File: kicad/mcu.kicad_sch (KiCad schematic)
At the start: 36 parts, among them J8 USB_C_Receptacle_USB2.0_14P, J9 Conn_01x03, SW1 SW_Push, SW2 SW_Push, U12 ESP32-S3-WROOM-1-N8R2

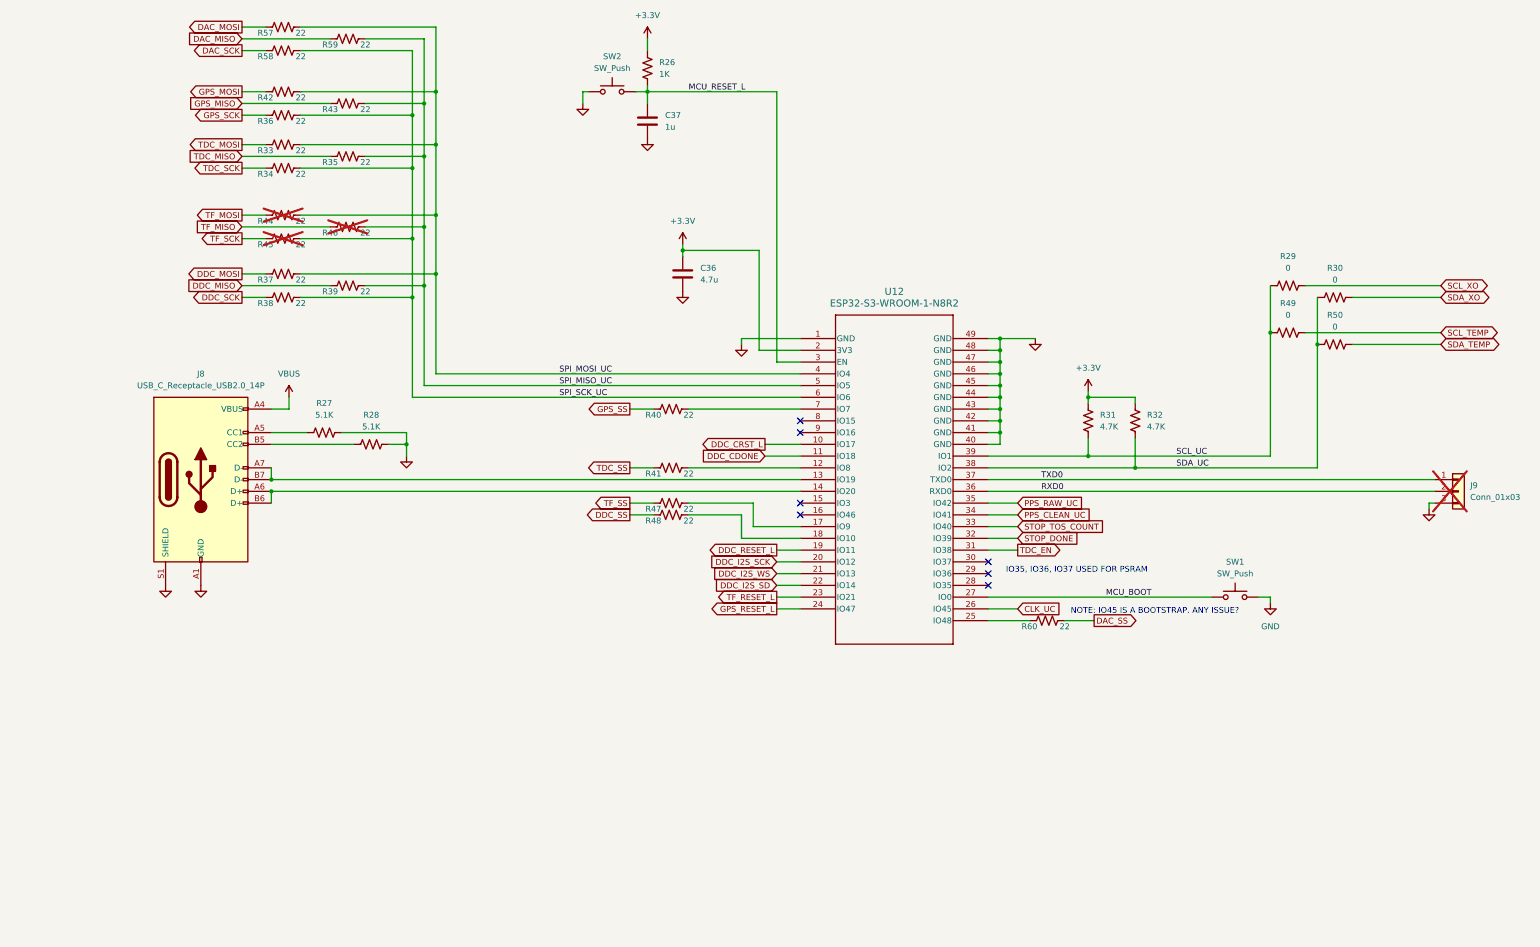
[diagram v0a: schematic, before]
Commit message: add lte radio and various fixes
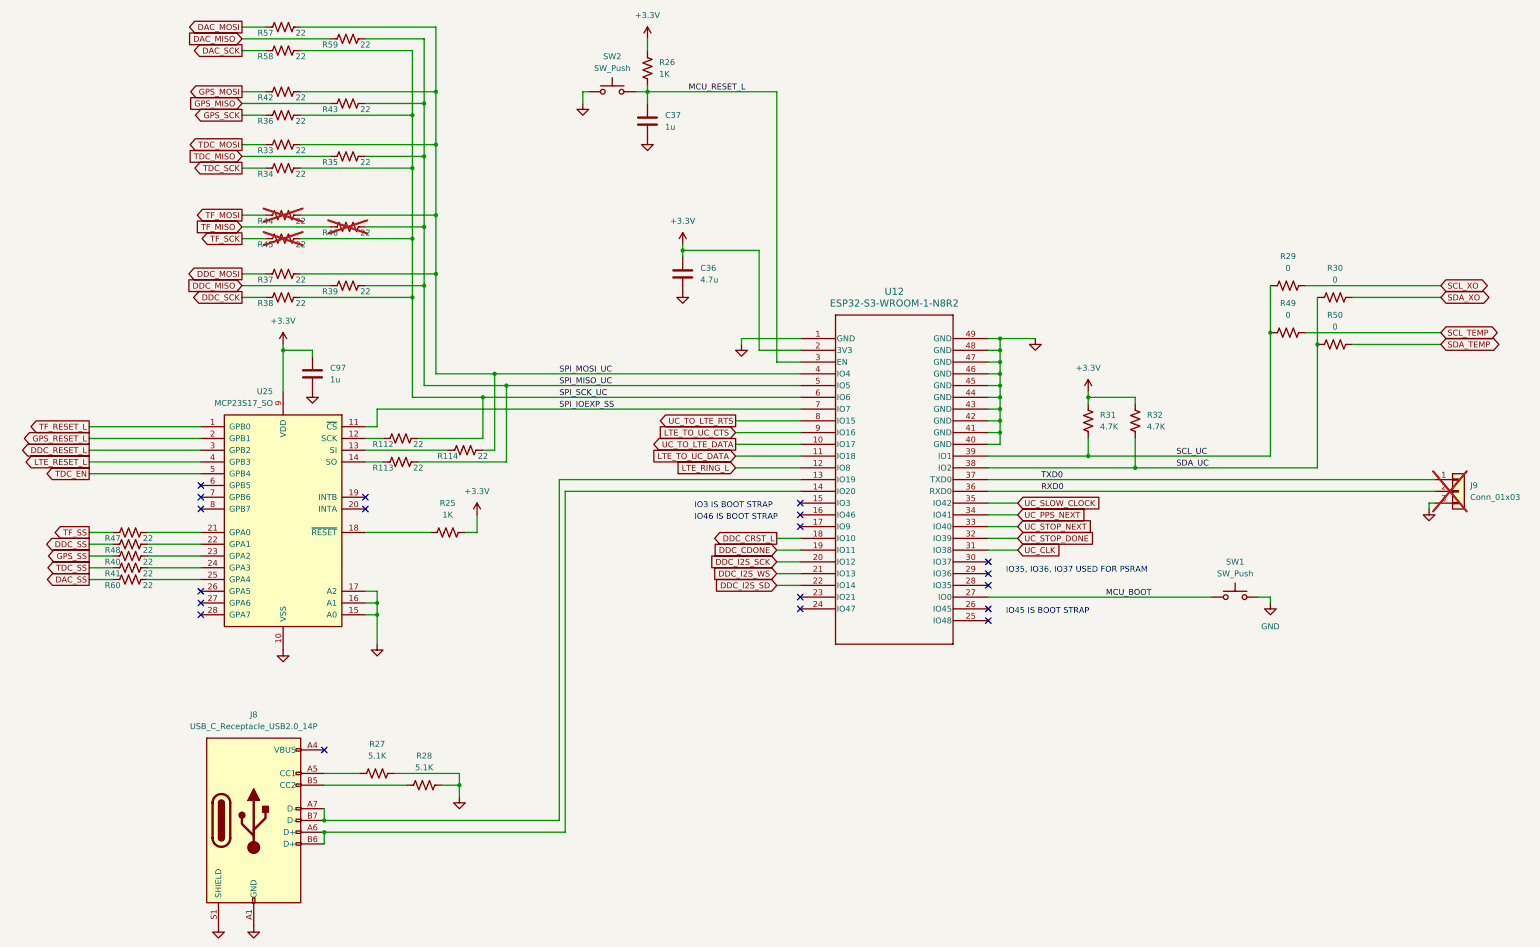
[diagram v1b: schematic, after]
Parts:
- added C97: 1u, symbol Device:C
- added R112, R113, R114: 22, symbol Device:R_US
- added R25: 1K, symbol Device:R_US
- added U25: MCP23S17_SO, Package_SO:SOIC-28W_7.5x17.9mm_P1.27mm, symbol Interface_Expansion:MCP23S17_SO
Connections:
- net +3.3V: now also C97.1, R25.2, U25.9 (VDD)
- net DDC_CDONE: now also U12.19 (IO11); no longer U12.11 (IO18)
- net DDC_CRST_L: now also U12.18 (IO10); no longer U12.10 (IO17)
- net DDC_RESET_L: now also U25.3 (GPB2); no longer U12.19 (IO11)
- net GND: now also C97.2, U25.10 (VSS), U25.15 (A0), U25.16 (A1), U25.17 (A2)
- net GPS_RESET_L: now also U25.2 (GPB1); no longer U12.24 (IO47)
- net SPI_MISO_UC: now also R113.2
- net SPI_MOSI_UC: now also R114.2
- net SPI_SCK_UC: now also R112.2
- net TDC_EN: now also U25.5 (GPB4); no longer U12.31 (IO38)
- net TF_RESET_L: now also U25.1 (GPB0); no longer U12.23 (IO21)
- net at R48.2: now also U25.22 (GPA1); no longer U12.18 (IO10)
- net at R41.2: now also U25.24 (GPA3); no longer U12.12 (IO8)
- net at U12.17 (IO9): no longer R47.2
- net at U12.25 (IO48): no longer R60.1
- net at R40.2: now also U25.23 (GPA2); no longer U12.7 (IO7)
- net UC_TO_LTE_RTS: now reaches U12.8 (IO15)
- net LTE_TO_UC_CTS: now reaches U12.9 (IO16)
- net CLK_UC: no longer names the net of U12.26 (IO45)
- net PPS_CLEAN_UC renamed UC_PPS_NEXT
- net PPS_RAW_UC renamed UC_SLOW_CLOCK
- net STOP_DONE renamed UC_STOP_DONE
- net STOP_TOS_COUNT renamed UC_STOP_NEXT
- net VBUS: no longer names the net of J8.A4 (VBUS), J8.A9 (VBUS), J8.B4 (VBUS), J8.B9 (VBUS)
- new net: R60.1, U25.25 (GPA4)
- new net: R112.1, U25.12 (SCK)
- new net: R47.2, U25.21 (GPA0)
- new net: R25.1, U25.18 (~{RESET})
- new net: R113.1, U25.14 (SO)
- new net: R114.1, U25.13 (SI)
- new net LTE_RESET_L: U25.4 (GPB3)
- new net LTE_RING_L: U12.12 (IO8)
- new net LTE_TO_UC_DATA: U12.11 (IO18)
- new net SPI_IOEXP_SS: U12.7 (IO7), U25.11 (~{CS})
- new net UC_CLK: U12.31 (IO38)
- new net UC_TO_LTE_DATA: U12.10 (IO17)
- no-connect marks 7 -> 19
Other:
- note added: "IO3 IS BOOT STRAP"
- note added: "IO45 IS BOOT STRAP"
- note added: "IO46 IS BOOT STRAP"
- note removed: "NOTE: IO45 IS A BOOTSTRAP. ANY ISSUE?"
- moved on the sheet: J8, R27, R28, R40, R41, R47, R48, R60

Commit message: assign footprints
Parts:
- C36, C37, C97: footprint (none) -> Capacitor_SMD:C_0603_1608Metric_Pad1.08x0.95mm_HandSolder
- J8: footprint (none) -> Connector_USB:USB_C_Receptacle_Molex_105450-0101
- J9: footprint (none) -> Connector_PinHeader_2.54mm:PinHeader_1x03_P2.54mm_Vertical
- R112, R113, R114, R25, R26, R27, R28, R29, R30, R31, R32, R33, R34, R35, R36, R37, R38, R39, R40, R41, R42, R43, R44, R45, R46, R47, R48, R49, R50, R57, R58, R59, R60: footprint (none) -> Resistor_SMD:R_0603_1608Metric_Pad0.98x0.95mm_HandSolder
- SW1, SW2: footprint (none) -> Button_Switch_SMD:SW_SPST_B3U-1000P
- U12: footprint ESP32-S3-WROOM-1_EXP -> bgelb_footprint:ESP32-S3-WROOM-1_EXP
